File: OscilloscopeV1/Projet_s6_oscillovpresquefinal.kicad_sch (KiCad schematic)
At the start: 33 parts, among them IC1 PGA849RGTR, J1 Conn_Coaxial, J2 Conn_01x06_Socket, J3 PILES_3AA, J4 Conn_01x05_Pin, SW1 SW_SPST, U1 MCP1826S, U3 AP2112K-3.3, U4 STM32L476RGTx

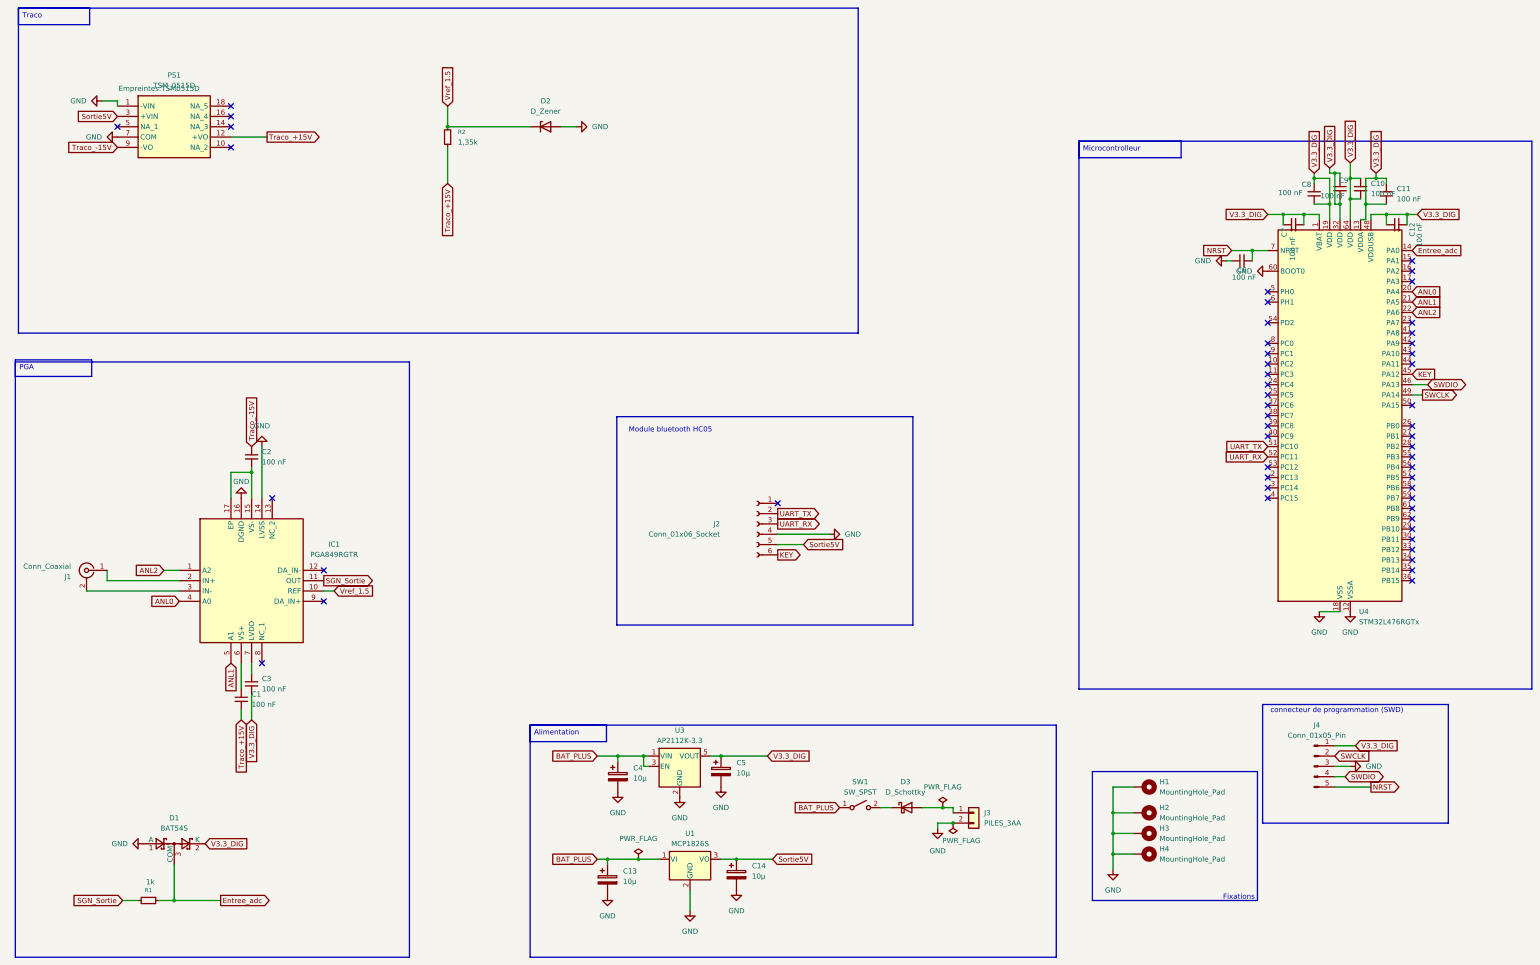
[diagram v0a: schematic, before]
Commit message: Start routing (#2)
* Point de départ du routage

* Merge pull request #1 from YounesAchb/End-routing

Add files via upload

* Add files via upload

routage du pcb the long way

* PCB Final

---------

Co-authored-by: YounesAchb <younes.achbad@ensea.fr>
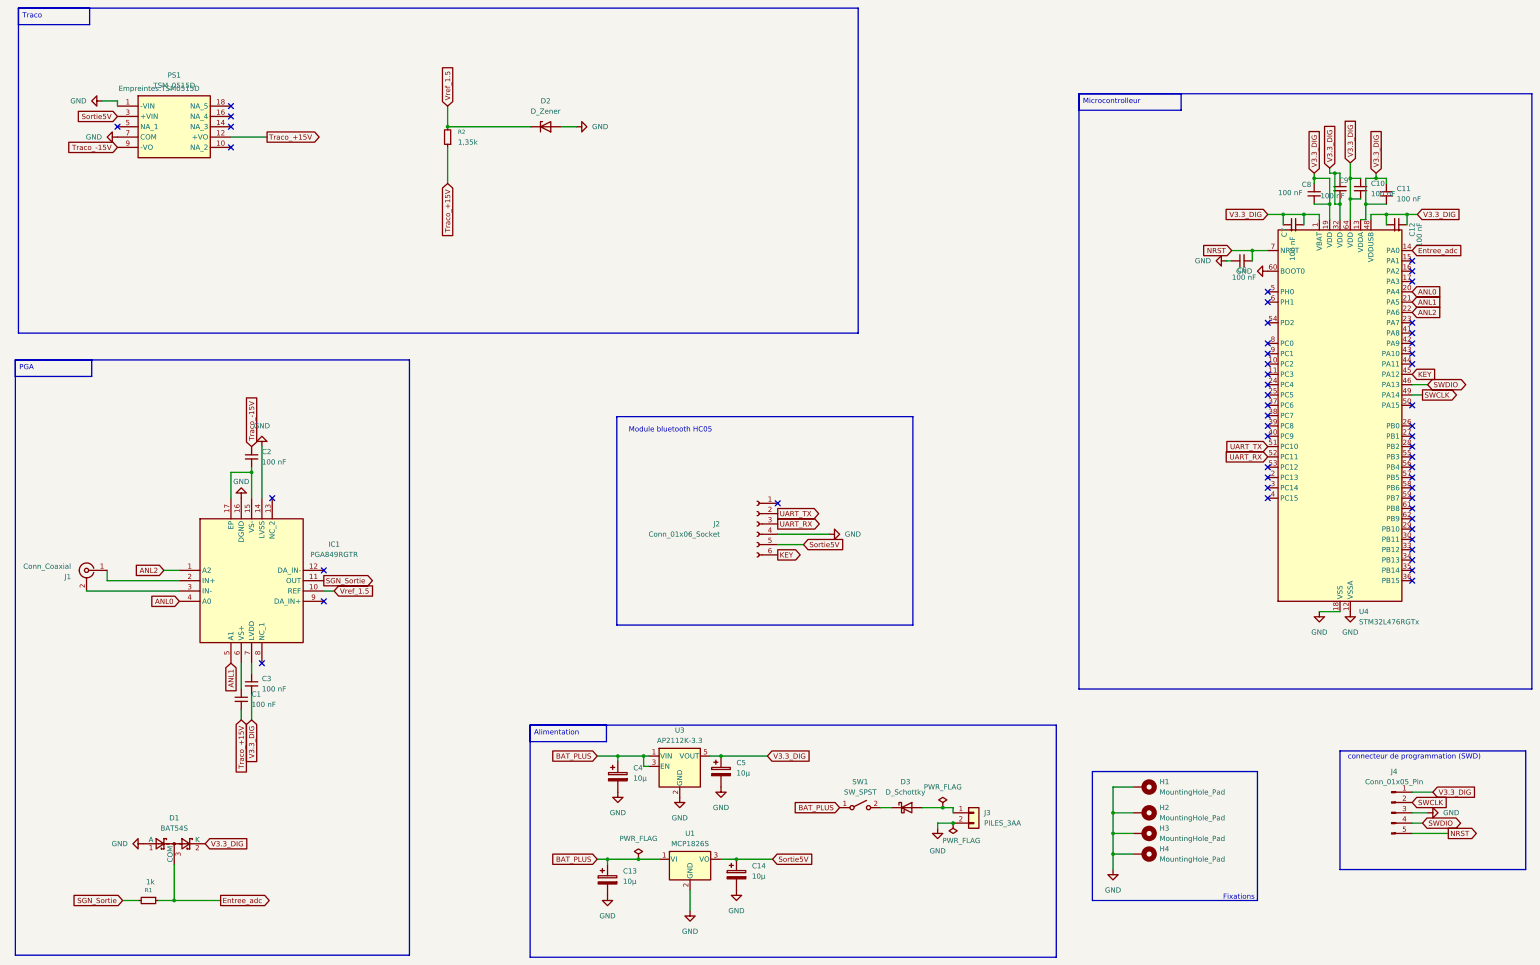
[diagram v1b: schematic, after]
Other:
- moved on the sheet: J4
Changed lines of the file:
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@@
 	)
 	(rectangle
-		(start 21.844 108.712)
-		(end 118.872 255.27)
+		(start 21.844 108.204)
+		(end 118.872 254.762)
 		(stroke
 			(width 0)
@@
 	)
 	(rectangle
-		(start 283.718 54.356)
+		(start 283.718 42.672)
 		(end 395.224 189.23)
 		(stroke
@@
 	)
 	(rectangle
-		(start 328.93 193.04)
-		(end 374.65 222.25)
+		(start 347.98 204.47)
+		(end 393.7 233.68)
 		(stroke
 			(width 0)
@@
 	(text "connecteur de programmation (SWD)"
 		(exclude_from_sim no)
-		(at 347.218 194.564 0)
+		(at 366.268 205.994 0)
 		(effects
 			(font
@@
 	(text_box "Microcontrolleur\n"
 		(exclude_from_sim no)
-		(at 283.718 54.356 0)
+		(at 283.718 42.672 0)
 		(size 25.146 4.064)
 		(margins 0.9525 0.9525 0.9525 0.9525)
@@
 	(wire
 		(pts
-			(xy 346.71 208.28) (xy 350.52 208.28)
+			(xy 365.76 219.71) (xy 369.57 219.71)
 		)
 		(stroke
@@
 	(wire
 		(pts
-			(xy 346.71 213.36) (xy 355.6 213.36)
+			(xy 365.76 224.79) (xy 374.65 224.79)
 		)
 		(stroke
@@
 	(wire
 		(pts
-			(xy 346.71 210.82) (xy 349.25 210.82)
+			(xy 365.76 222.25) (xy 368.3 222.25)
 		)
 		(stroke
@@
 	(wire
 		(pts
-			(xy 346.71 203.2) (xy 351.79 203.2)
+			(xy 365.76 214.63) (xy 370.84 214.63)
 		)
 		(stroke
@@
 	(global_label "NRST"
 		(shape output)
-		(at 355.6 213.36 0)
+		(at 374.65 224.79 0)
 		(fields_autoplaced yes)
 		(effects
@@
 		)
 		(property "Intersheetrefs" "${INTERSHEET_REFS}"
-			(at 363.3628 213.36 0)
+			(at 382.4128 224.79 0)
 			(effects
 				(font
@@
 	(global_label "SWDIO"
 		(shape bidirectional)
-		(at 349.25 210.82 0)
+		(at 368.3 222.25 0)
 		(fields_autoplaced yes)
 		(effects
@@
 		)
 		(property "Intersheetrefs" "${INTERSHEET_REFS}"
-			(at 359.2127 210.82 0)
+			(at 378.2627 222.25 0)
 			(effects
 				(font
@@
 	(global_label "V3.3_DIG"
 		(shape input)
-		(at 351.79 203.2 0)
+		(at 370.84 214.63 0)
 		(fields_autoplaced yes)
 		(effects
@@
 		)
 		(property "Intersheetrefs" "${INTERSHEET_REFS}"
-			(at 363 203.2 0)
+			(at 382.05 214.63 0)
 			(effects
 				(font
@@
 	(global_label "SWCLK"
 		(shape input)
-		(at 346.71 205.74 0)
+		(at 365.76 217.17 0)
 		(fields_autoplaced yes)
 		(effects
@@
 		)
 		(property "Intersheetrefs" "${INTERSHEET_REFS}"
-			(at 355.9242 205.74 0)
+			(at 374.9742 217.17 0)
 			(effects
 				(font
@@
 	(symbol
 		(lib_id "power:GND")
-		(at 350.52 208.28 90)
+		(at 369.57 219.71 90)
 		(unit 1)
 		(exclude_from_sim no)
@@
 		(fields_autoplaced yes)
 		(property "Reference" "#PWR018"
-			(at 356.87 208.28 0)
+			(at 375.92 219.71 0)
 			(effects
 				(font
@@
 		)
 		(property "Value" "GND"
-			(at 354.33 208.2799 90)
+			(at 373.38 219.7099 90)
 			(effects
 				(font
@@
 		)
 		(property "Footprint" ""
-			(at 350.52 208.28 0)
+			(at 369.57 219.71 0)
 			(effects
 				(font
@@
 		)
 		(property "Datasheet" ""
-			(at 350.52 208.28 0)
+			(at 369.57 219.71 0)
 			(effects
 				(font
@@
 		)
 		(property "Description" "Power symbol creates a global label with name \"GND\" , ground"
-			(at 350.52 208.28 0)
+			(at 369.57 219.71 0)
 			(effects
 				(font
@@
 	(symbol
 		(lib_id "Connector:Conn_01x05_Pin")
-		(at 341.63 208.28 0)
+		(at 360.68 219.71 0)
 		(unit 1)
 		(exclude_from_sim no)
@@
 		(fields_autoplaced yes)
 		(property "Reference" "J4"
-			(at 342.265 198.12 0)
+			(at 361.315 209.55 0)
 			(effects
 				(font
@@
 		)
 		(property "Value" "Conn_01x05_Pin"
-			(at 342.265 200.66 0)
+			(at 361.315 212.09 0)
 			(effects
 				(font
@@
 		)
 		(property "Footprint" "Connector_PinHeader_2.54mm:PinHeader_1x05_P2.54mm_Vertical"
-			(at 341.63 208.28 0)
+			(at 360.68 219.71 0)
 			(effects
 				(font
@@
 		)
 		(property "Datasheet" "~"
-			(at 341.63 208.28 0)
+			(at 360.68 219.71 0)
 			(effects
 				(font
@@
 		)
 		(property "Description" "Generic connector, single row, 01x05, script generated"
-			(at 341.63 208.28 0)
+			(at 360.68 219.71 0)
 			(effects
 				(font

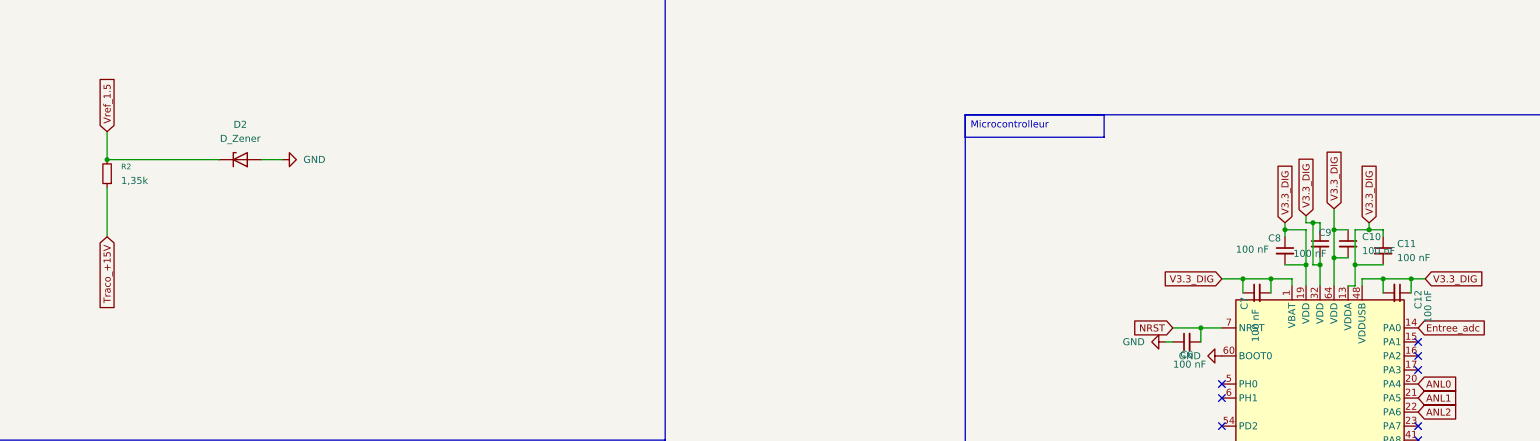
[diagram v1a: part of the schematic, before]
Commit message: Add files via upload
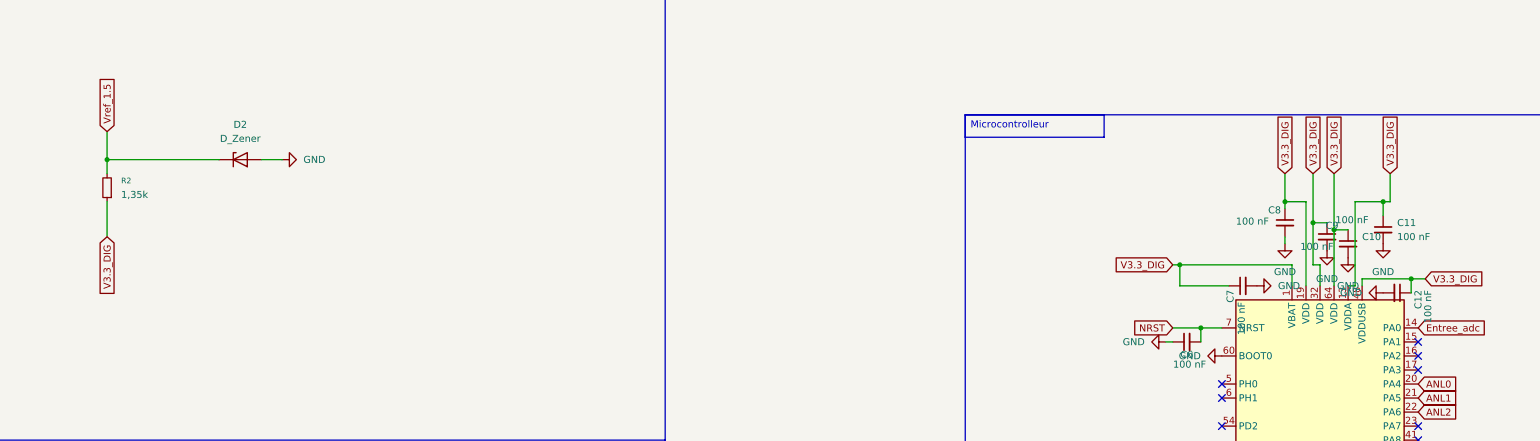
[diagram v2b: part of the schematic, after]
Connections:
- net GND: now also C10.2, C11.2, C12.2, C7.2, C8.2, C9.2
- net Traco_+15V: no longer R2.1
- net V3.3_DIG: now also R2.1; no longer C10.2, C11.2, C12.2, C7.2, C8.2, C9.2
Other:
- moved on the sheet: C11, C7, C8, C9, R2
